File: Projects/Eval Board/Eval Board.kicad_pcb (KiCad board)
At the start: 2 copper layers, 50.8 x 33.5 mm, 34 parts, among them J1 I OUT, J2 Q OUT, J3 LO, J4 RF, U1 LTC5584

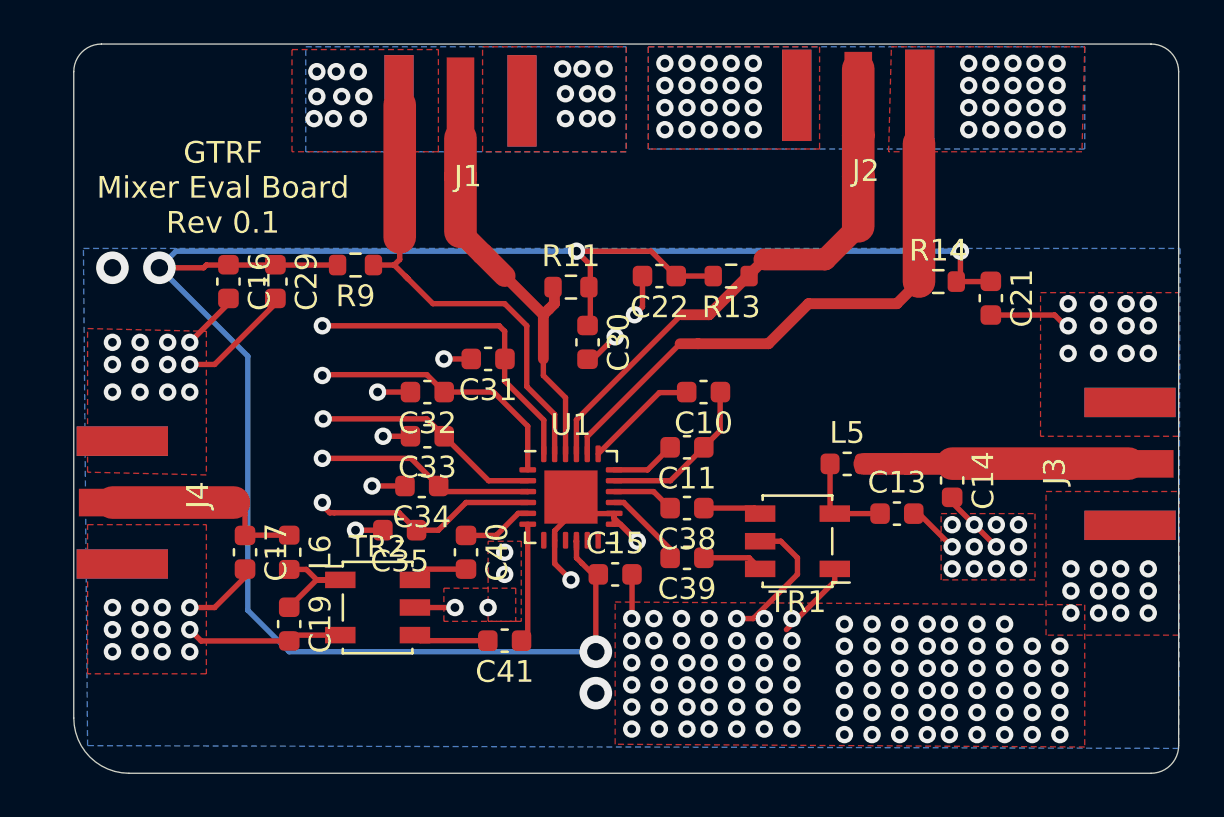
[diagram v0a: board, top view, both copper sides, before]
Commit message: Version 2
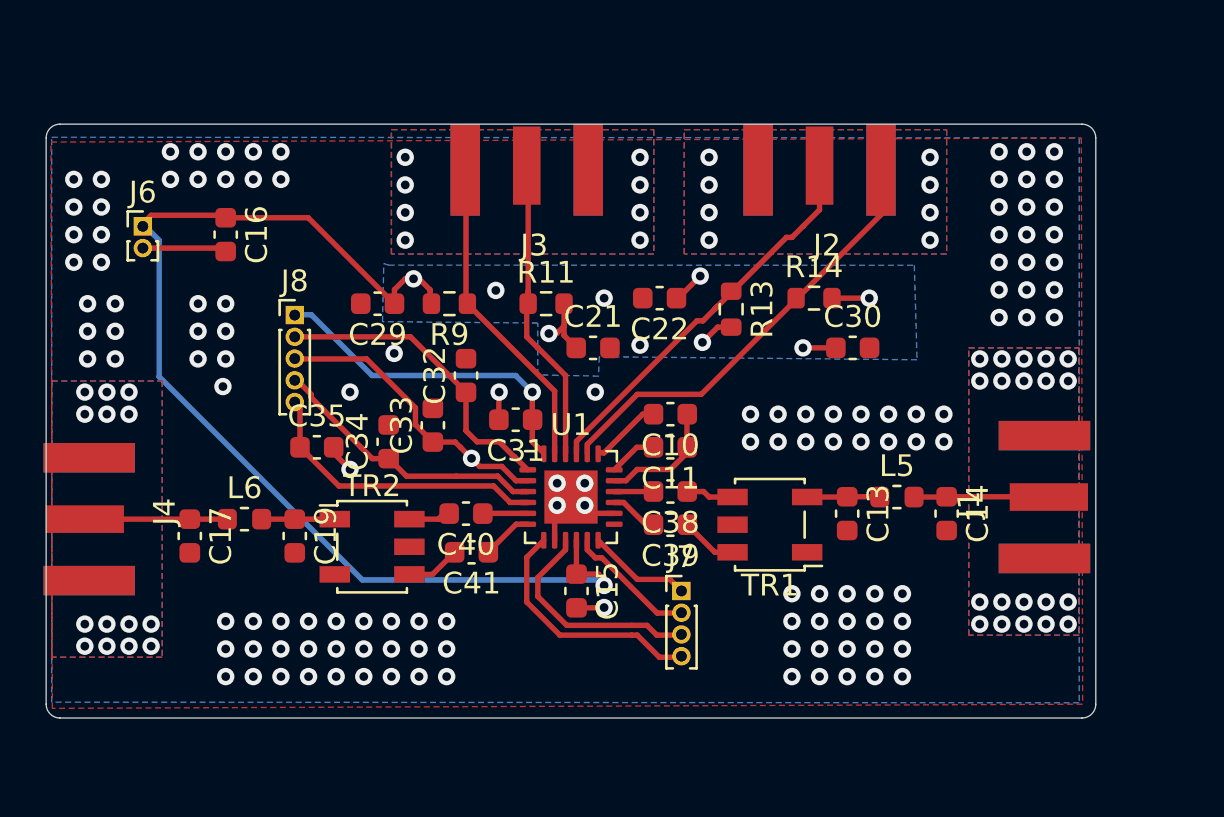
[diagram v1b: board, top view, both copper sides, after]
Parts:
- added J6: Conn_01x02, Connector_PinHeader_1.00mm:PinHeader_1x02_P1.00mm_Vertical, F.Cu at (175.9, 70.1)
- added J7: Conn_01x04, Connector_PinHeader_1.00mm:PinHeader_1x04_P1.00mm_Vertical, F.Cu at (200.7, 86.9)
- added J8: Conn_01x05, Connector_PinHeader_1.00mm:PinHeader_1x05_P1.00mm_Vertical, F.Cu at (182.9, 74.2)
- J1: value I OUT -> LO; footprint Kevin Library:SAMTEC_SMA-J-P-H-ST-EM1 -> AdditionalLibs:SAMTEC_SMA-J-P-H-ST-EM1
- J2: footprint Kevin Library:SAMTEC_SMA-J-P-H-ST-EM1 -> AdditionalLibs:SAMTEC_SMA-J-P-H-ST-EM1
- J3: value LO -> I Out; footprint Kevin Library:SAMTEC_SMA-J-P-H-ST-EM1 -> AdditionalLibs:SAMTEC_SMA-J-P-H-ST-EM1
- J4: value RF -> Q OUT; footprint Kevin Library:SAMTEC_SMA-J-P-H-ST-EM1 -> AdditionalLibs:SAMTEC_SMA-J-P-H-ST-EM1
- moved J1 32.7 mm to (217.6, 82.5), turned to 90 degrees
- moved J3 31.1 mm to (193.5, 67.3), turned to 180 degrees
- moved C21 18.4 mm to (196.6, 75.7), turned to 0 degrees
- moved C30 12.2 mm to (208.5, 75.7), turned to 0 degrees
- moved R14 5.77 mm to (206.8, 73.4)
- moved C35 5.39 mm to (183.9, 80.3), turned to 0 degrees
- moved C29 4.81 mm to (186.7, 73.7), turned to 180 degrees
- moved R9 4.67 mm to (190.0, 73.7)
- moved C41 4.34 mm to (191.0, 85.1)
- moved C19 4.06 mm to (182.9, 84.3)
- moved J2 3.86 mm to (207.0, 67.3)
- moved C31 3.07 mm to (193.0, 79.0)
- moved TR2 2.81 mm to (186.4, 84.8)
- moved L5 2.75 mm to (210.6, 82.5)
- moved C17 2.65 mm to (178.1, 84.3)
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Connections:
- net DCOI renamed /DCOI
- net DCOQ renamed /DCOQ
- net IP2I renamed /IP21
- net IP2Q renamed /IP2Q
- net Net-(C17-Pad1) renamed /RF
- net Net-(J2-Pad1) renamed /Q+
- net Net-(J2-Pad2_1) renamed /Q-
- C14 pad 1: Net-(C14-Pad1) -> /LO
- J1 pad 1: Net-(J1-Pad1) -> /LO
- J1 pad 2_1: Net-(J1-Pad2_1) -> GND
- J1 pad 2_2: Net-(J1-Pad2_1) -> GND
- J1 pad 3_1: Net-(J1-Pad2_1) -> GND
- J1 pad 3_2: Net-(J1-Pad2_1) -> GND
- J3 pad 1: Net-(C14-Pad1) -> /I+
- J3 pad 2_1: GND -> /I-
- J3 pad 2_2: GND -> /I-
- J3 pad 3_1: GND -> /I-
- J3 pad 3_2: GND -> /I-
- L5 pad 2: Net-(C14-Pad1) -> /LO
- R11 pad 1: Net-(J1-Pad1) -> /I+
- R9 pad 1: Net-(J1-Pad2_1) -> /I-
- U1 pad 22: Net-(J1-Pad1) -> /I+
- U1 pad 23: Net-(J1-Pad2_1) -> /I-
- U1 pad 25: (no net) -> GND
- U1 pad 9: Net-(U1-Pad9) -> Vbias
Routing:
- net GND: track 61.1 -> 10.5 mm, vias 169 -> 161
- net VCC: track 99.5 -> 61.3 mm, vias 4 -> 8
- net Net-(J1-Pad1): track 23.1 -> 0.00 mm
- net Net-(J1-Pad2_1): track 22.8 -> 0.00 mm, vias 18 -> 0
- net /I-: track 0.00 -> 13.4 mm, vias 0 -> 8
- net /I+: track 0.00 -> 12.6 mm
- net Net-(C14-Pad1): track 12.2 -> 0.00 mm
- net EN: track 0.00 -> 11.3 mm
- net Vbias: track 0.00 -> 10.5 mm
- net /Q+: track 25.7 -> 19.1 mm
- net /LO: track 0.00 -> 6.20 mm
- net EDC: track 0.00 -> 5.97 mm
- net /Q-: track 27.6 -> 21.6 mm, vias 40 -> 8
- net EIP2: track 0.00 -> 4.80 mm
- net /DCOI: track 10.1 -> 13.3 mm, vias 1 -> 0
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- added copper zone on B.Cu, net /I-
- added copper zone on F.Cu, net /I-
- added copper zone on B.Cu, net VCC
- removed copper zone on B.Cu, net Net-(J1-Pad2_1)
- removed copper zone on F.Cu, net Net-(J1-Pad2_1)
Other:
- board size 50.8 x 33.5 mm -> 48.3 x 27.3 mm
- board text removed: "GTRF Mixer Eval Board Rev 0.1"
